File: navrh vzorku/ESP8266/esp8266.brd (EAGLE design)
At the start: 160 x 100 mm, 23 parts

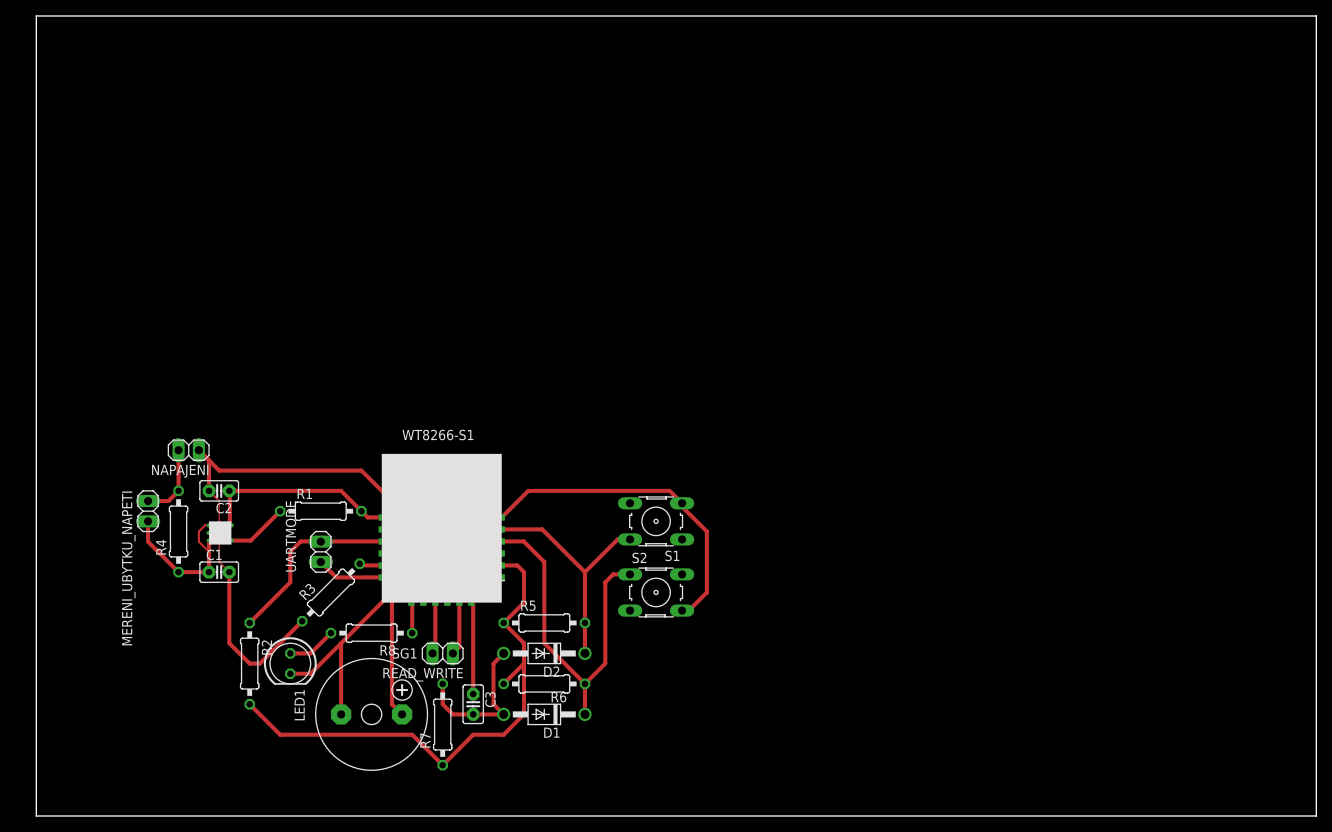
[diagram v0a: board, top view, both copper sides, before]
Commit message: Plosne spoje
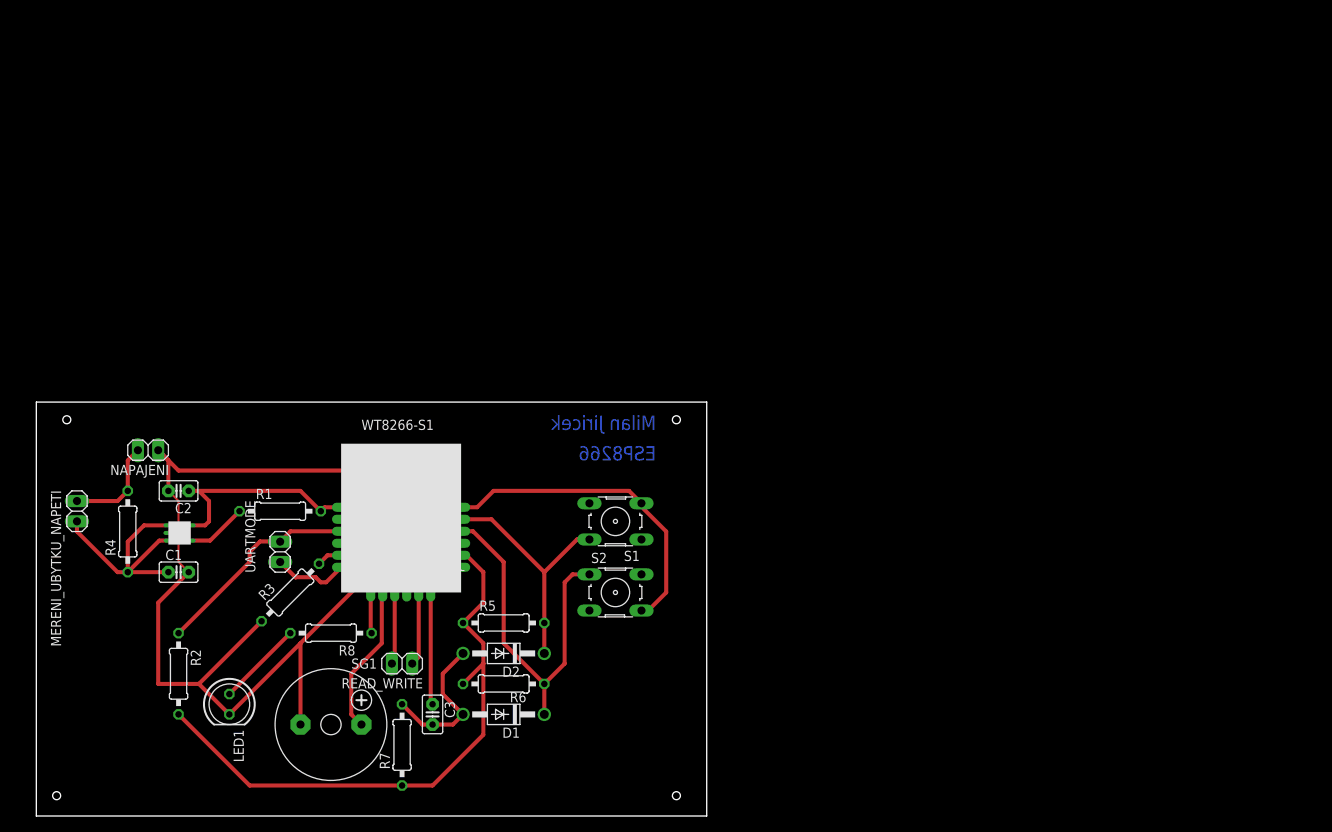
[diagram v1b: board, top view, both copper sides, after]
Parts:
- moved LED1 9.16 mm to (24.1, 14.0)
- moved R2 8.98 mm to (17.8, 17.8)
- moved MERENI_UBYTKU_NAPETI 8.89 mm to (5.08, 38.1)
- moved R4 6.35 mm to (11.4, 35.6)
- moved R7 5.68 mm to (45.7, 8.89)
- moved C3 5.24 mm to (49.5, 12.7)
- moved READ_WRITE 5.24 mm to (45.7, 19.1)
- moved SG1 5.24 mm to (36.8, 11.4)
- moved U$1 5.24 mm to (38.1, 27.9)
- moved R1 5.08 mm to (30.5, 38.1)
- moved UARTMODE 5.08 mm to (30.5, 33.0)
- moved NAPAJENI 5.08 mm to (14.0, 45.7)
- moved C1 5.08 mm to (17.8, 30.5)
- moved C2 5.08 mm to (17.8, 40.6)
- moved D1 5.08 mm to (58.4, 12.7)
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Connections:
- removed net N$18: LED1.K, SG1.-, U$1.GND2
- removed net N$6: C1.2, C2.2, NAPAJENI.1, R3.1, S1.3, S2.4, U$1.GND, U$2.GND
- new net GND: C1.2, C2.2, LED1.K, NAPAJENI.1, R3.1, S1.3, S2.4, SG1.-, U$1.GND, U$1.GND2, U$2.GND
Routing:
- net GND: track 0.00 -> 180.4 mm
- net N$6: track 121.6 -> 0.00 mm
- net N$18: track 35.8 -> 0.00 mm
- net N$1: track 20.6 -> 31.1 mm
- net N$2: track 108.9 -> 118.7 mm
- net N$16: track 6.13 -> 10.8 mm
- net N$3: track 23.0 -> 26.4 mm
- net N$10: track 9.42 -> 12.5 mm
- net N$11: track 11.5 -> 14.1 mm
- net N$5: track 6.49 -> 9.03 mm
- net N$7: track 6.69 -> 9.23 mm
- net N$17: track 21.2 -> 18.7 mm
- net N$15: track 3.86 -> 5.13 mm
- net N$8: track 8.42 -> 9.49 mm
- net N$9: track 2.85 -> 3.50 mm
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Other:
- board size 160 x 100 mm -> 83.8 x 51.7 mm
- board text added: "ESP8266"
- board text added: "Milan Jiricek"

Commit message: Finalni verze
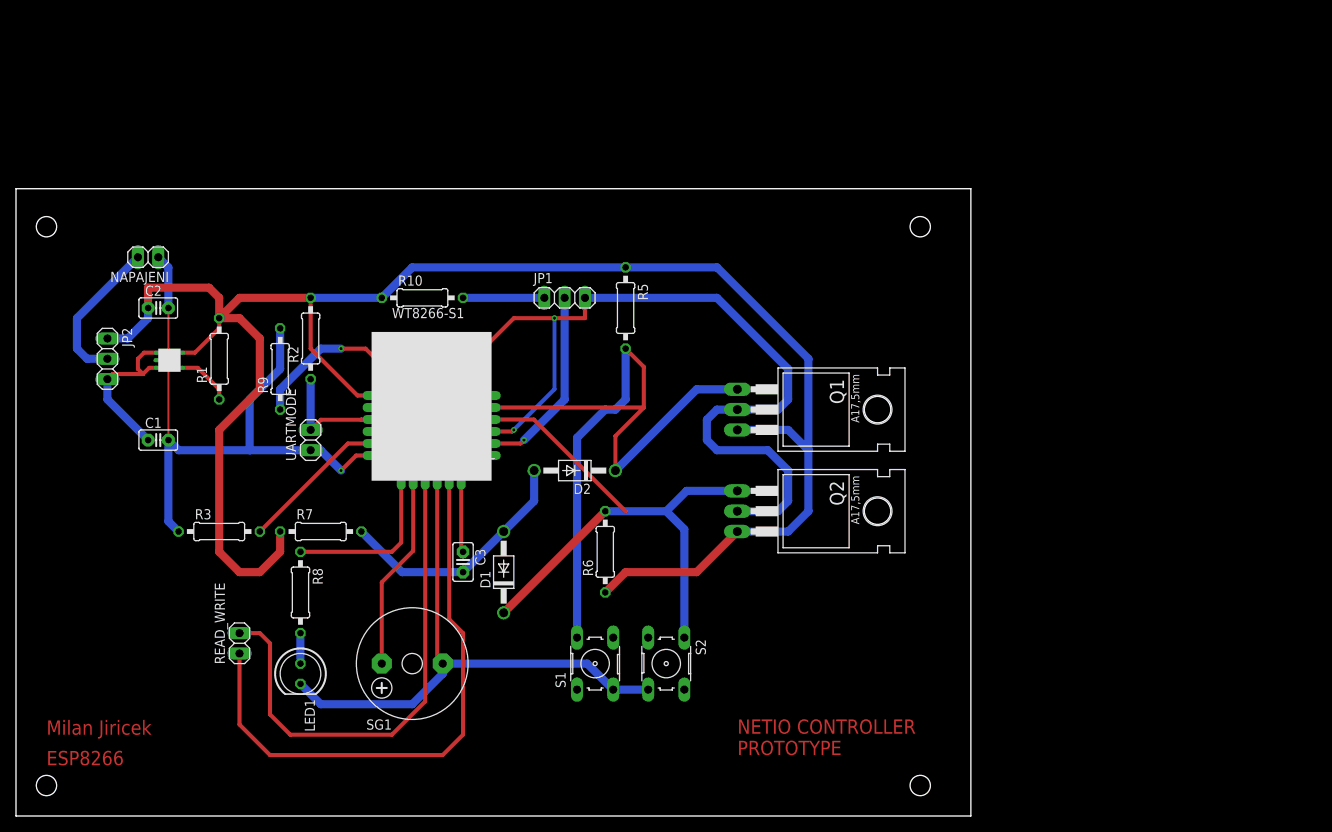
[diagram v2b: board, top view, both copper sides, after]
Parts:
- removed MERENI_UBYTKU_NAPETI: (no value), pinhead:1X02
- removed R4: 10, rcl:0207/10
- added JP1, JP2: (no value), pinhead:1X03
- added Q1, Q2: IRF4905, transistor-power:TO220BH
- added R10, R9: 2k, rcl:0207/10
- R2, R5, R6, R7: value 10k -> 2k
- moved R2 45.0 mm to (34.3, 59.7), turned to 90 degrees
- moved R5 42.2 mm to (73.7, 63.5), turned to 270 degrees
- moved R7 28.5 mm to (35.6, 35.6), turned to 0 degrees
- moved D2 24.5 mm to (67.3, 43.2)
- moved NAPAJENI 24.1 mm to (14.0, 69.8)
- moved C2 23.0 mm to (15.2, 63.5), turned to 0 degrees
- moved U$2 21.6 mm to (15.2, 58.4)
- moved R6 20.8 mm to (71.1, 33.0), turned to 90 degrees
- moved R1 20.5 mm to (22.9, 57.1), turned to 90 degrees
- moved READ_WRITE 20.5 mm to (25.4, 21.6), turned to 90 degrees
- moved C3 19.4 mm to (53.3, 31.8)
- moved S1 18.0 mm to (69.8, 19.1), turned to 90 degrees
- moved D1 17.8 mm to (58.4, 30.5), turned to 90 degrees
- moved C1 16.7 mm to (15.2, 47.0)
- moved UARTMODE 14.5 mm to (34.3, 47.0)
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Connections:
- removed net N$10: MERENI_UBYTKU_NAPETI.1, NAPAJENI.2, R4.2
- removed net N$8: U$1.GND1, UARTMODE.1
- new net N$18: JP1.3, Q1.D, Q2.D, R9.1, U$1.IO16
- new net N$19: JP1.2, U$1.EN
- new net N$20: JP1.1, R10.2
- new net N$6: C2.1, JP2.1, Q1.S, Q2.S, R1.2, R10.1, R2.2, R5.1, R6.1, R7.1, U$1.3.3V, U$2.OUT
- net GND: now also R9.2, S2.3, U$1.GND1, UARTMODE.1
- net N$1: now also JP2.3; no longer MERENI_UBYTKU_NAPETI.2, R4.1
- net N$12: now also Q2.G
- net N$13: now also Q1.G
- net N$2: now also JP2.2, NAPAJENI.2; no longer C2.1, R1.2, R2.2, R5.1, R6.1, R7.1, U$1.3.3V, U$1.EN, U$2.OUT
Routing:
- net N$6: track 0.00 -> 232.3 mm
- net N$18: track 0.00 -> 141.3 mm, vias 0 -> 3
- net N$2: track 118.7 -> 18.9 mm
- net N$13: track 30.6 -> 95.5 mm
- net N$7: track 9.23 -> 71.9 mm
- net N$5: track 9.03 -> 63.0 mm
- net N$12: track 45.3 -> 73.8 mm
- net N$19: track 0.00 -> 24.1 mm, vias 0 -> 1
- net N$15: track 5.13 -> 20.8 mm
- net N$9: track 3.50 -> 18.5 mm
- net N$10: track 12.5 -> 0.00 mm
- net N$14: track 18.9 -> 31.2 mm
- net N$3: track 26.4 -> 14.5 mm
- net N$20: track 0.00 -> 10.2 mm
- net N$1: track 31.1 -> 21.5 mm
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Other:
- board size 83.8 x 51.7 mm -> 119.4 x 78.4 mm
- board text added: "NETIO CONTROLLER PROTOTYPE"
